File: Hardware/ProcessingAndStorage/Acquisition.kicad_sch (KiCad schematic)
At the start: 19 parts, among them J1 Conn_Coaxial, J2 Conn_Coaxial, J3 Conn_Coaxial, J4 Conn_Coaxial, J8 DE9_Plug_MountingHoles, Q1 BC848, Q2 BC848, Q3 BC848, Q4 BC848

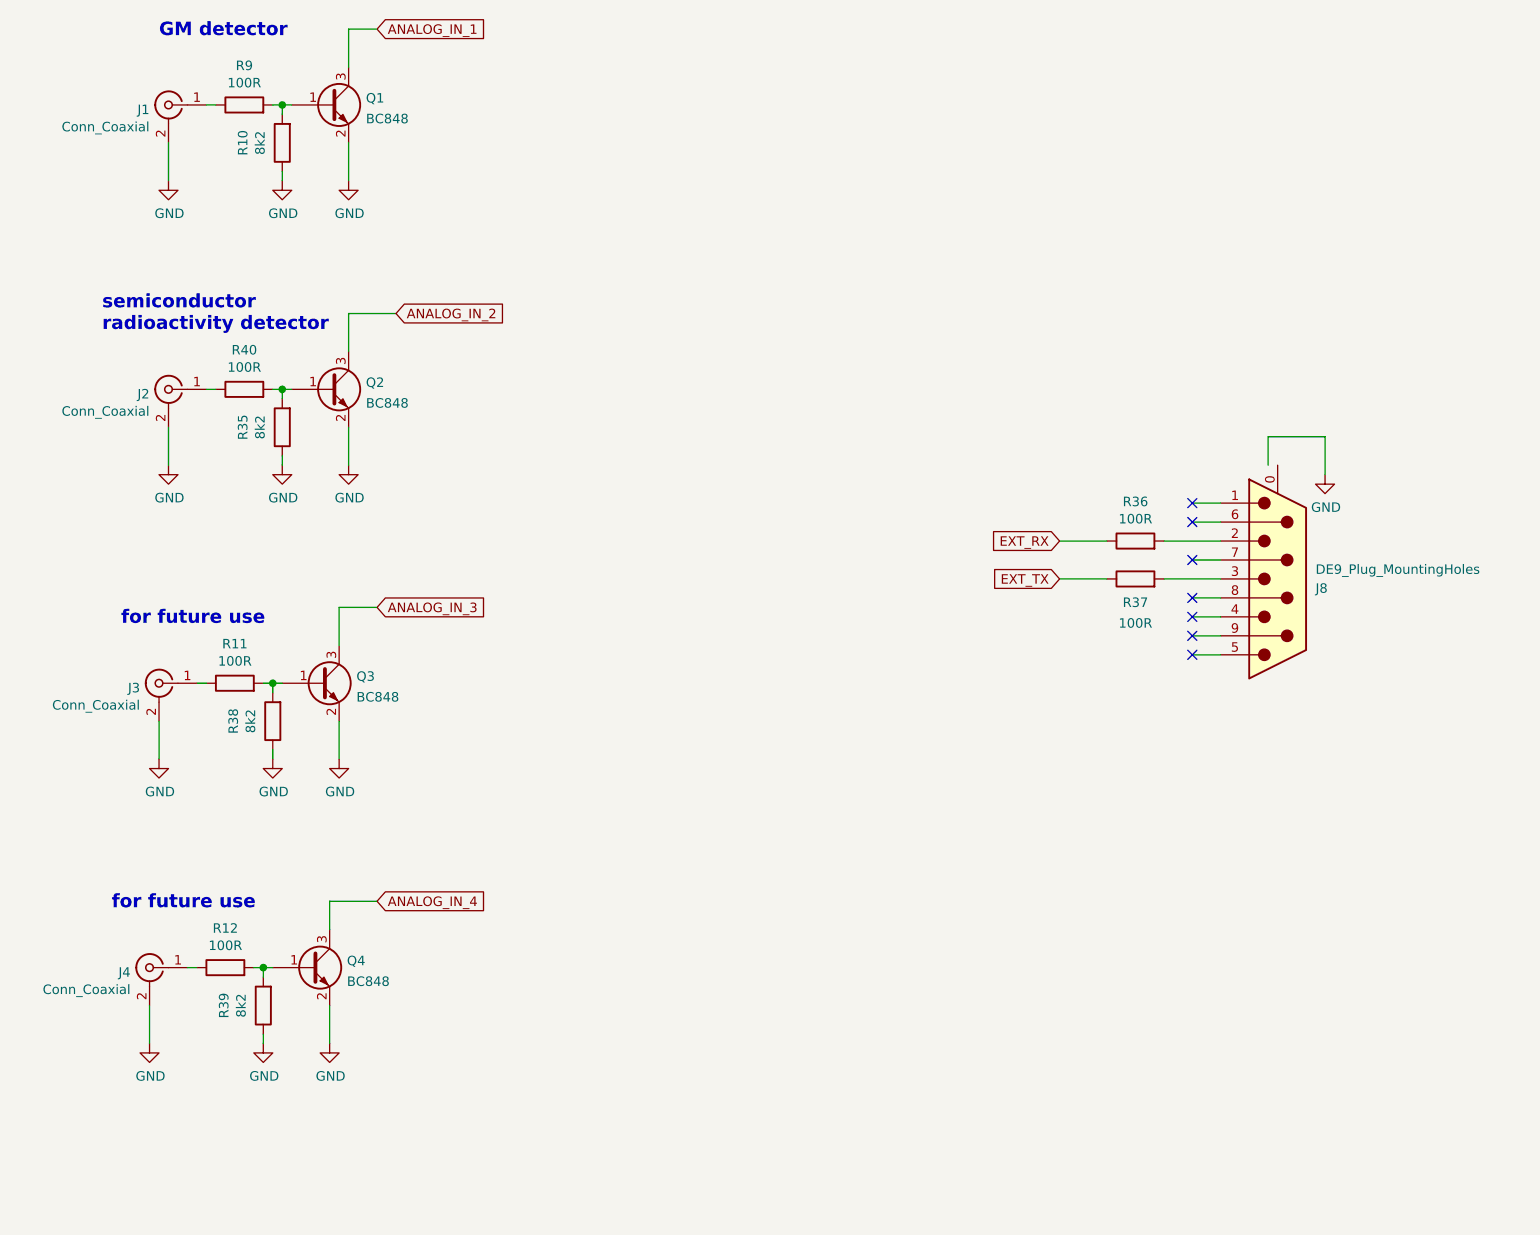
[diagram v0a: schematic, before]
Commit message: fix #148, fix #146, fix #151, fix #157
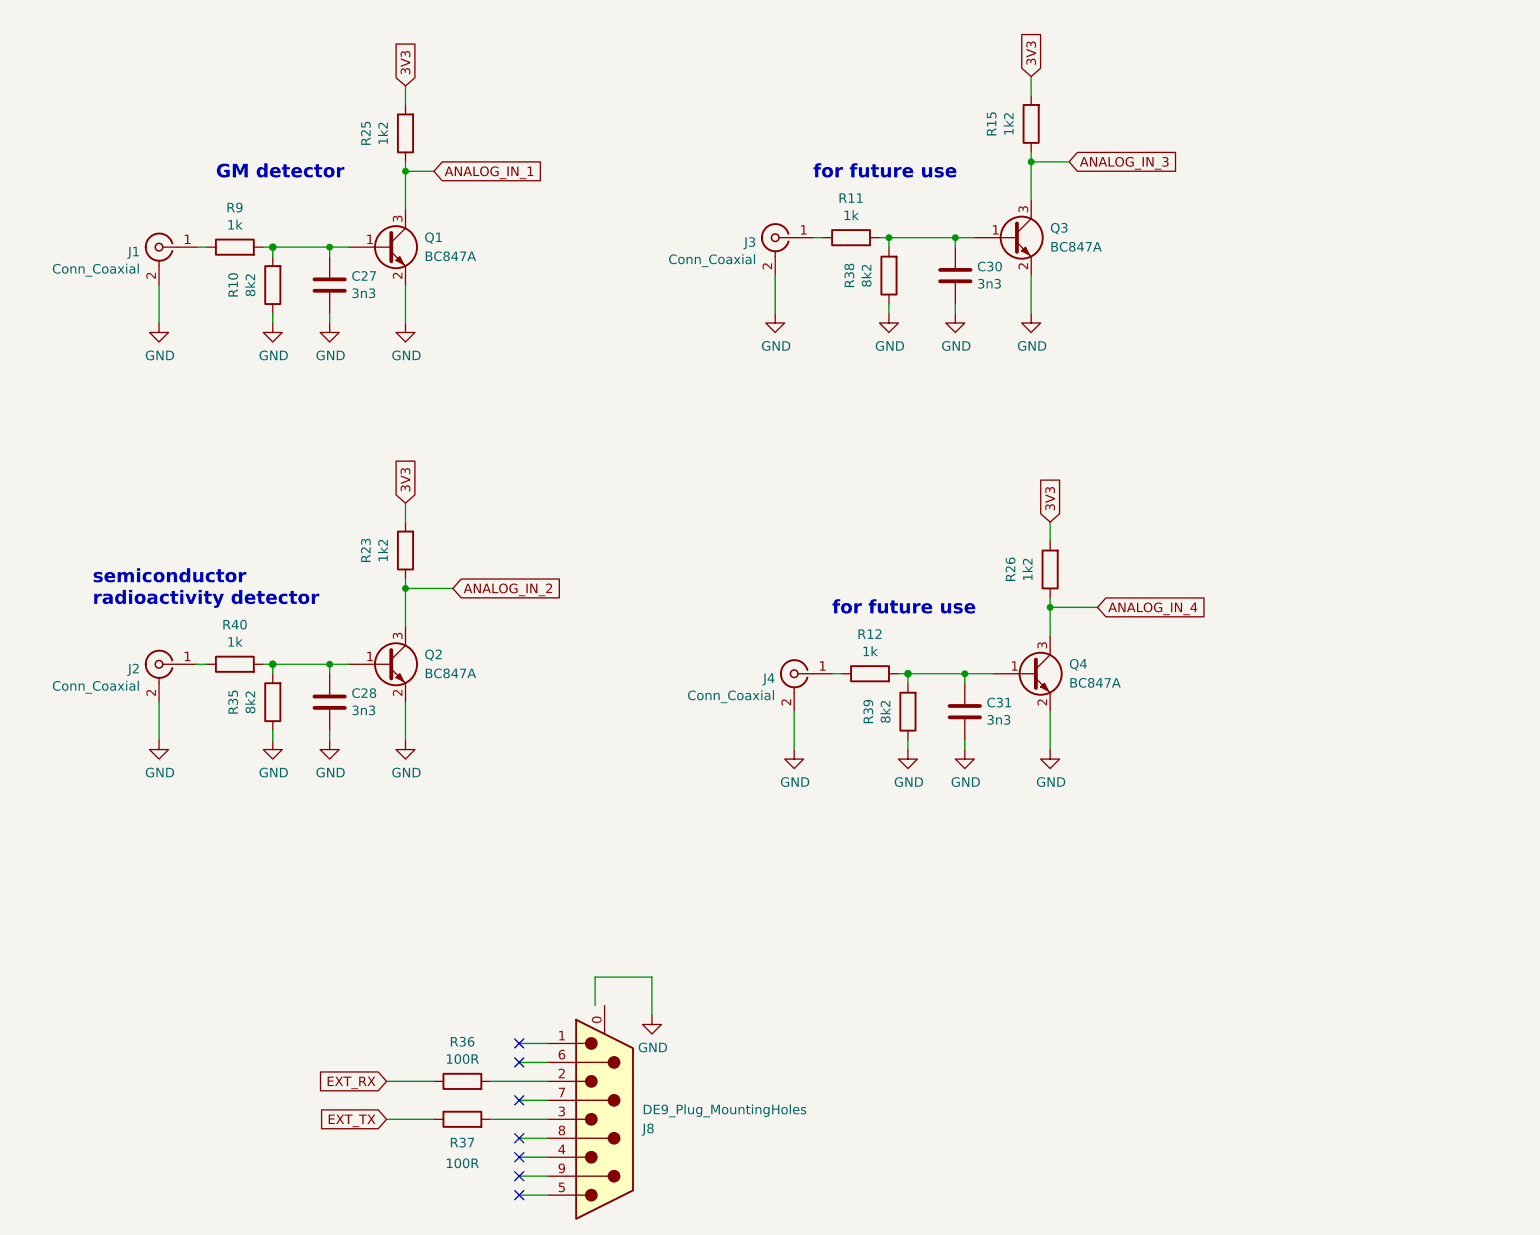
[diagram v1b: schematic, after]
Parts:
- added C27, C28, C30, C31: 3n3, Capacitor_SMD:C_0805_2012Metric, symbol Device:C
- added R15, R23, R25, R26: 1k2, Resistor_SMD:R_0805_2012Metric, symbol Device:R
- Q1, Q2, Q3, Q4: value BC848 -> BC847A
- R11, R12, R40, R9: value 100R -> 1k
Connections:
- net ANALOG_IN_1: now also R25.1
- net ANALOG_IN_2: now also R23.1
- net ANALOG_IN_3: now also R15.1
- net ANALOG_IN_4: now also R26.1
- net GND: now also C27.2, C28.2, C30.2, C31.2
- net at Q1.1 (B), R10.2, R9.2: now also C27.1
- net at Q3.1 (B), R11.2, R38.2: now also C30.1
- net at Q4.1 (B), R12.2, R39.2: now also C31.1
- net at Q2.1 (B), R35.2, R40.2: now also C28.1
- new net 3V3: R15.2, R23.2, R25.2, R26.2
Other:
- moved on the sheet: J1, J2, J3, J4, J8, Q1, Q2, Q3, Q4, R10, R11, R12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
